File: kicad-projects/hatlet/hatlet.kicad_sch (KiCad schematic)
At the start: 29 parts, among them J1 USB Header, J2 SWD, SW1 BOOTSEL, U1 AMS1117-3.3, U2 RP2040, U3 W25Q128JVS

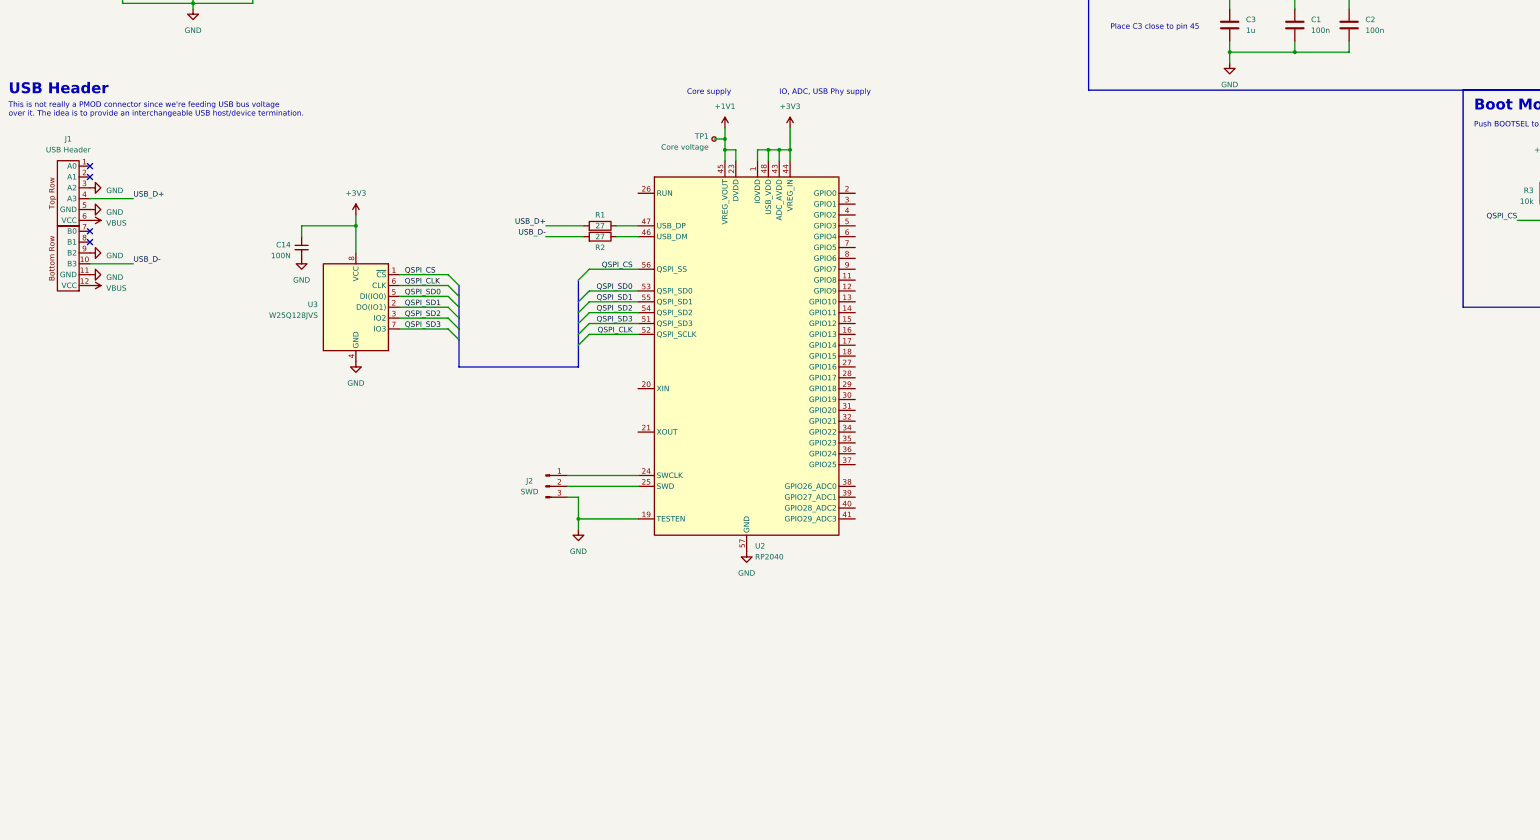
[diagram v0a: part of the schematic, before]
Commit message: Add crystal
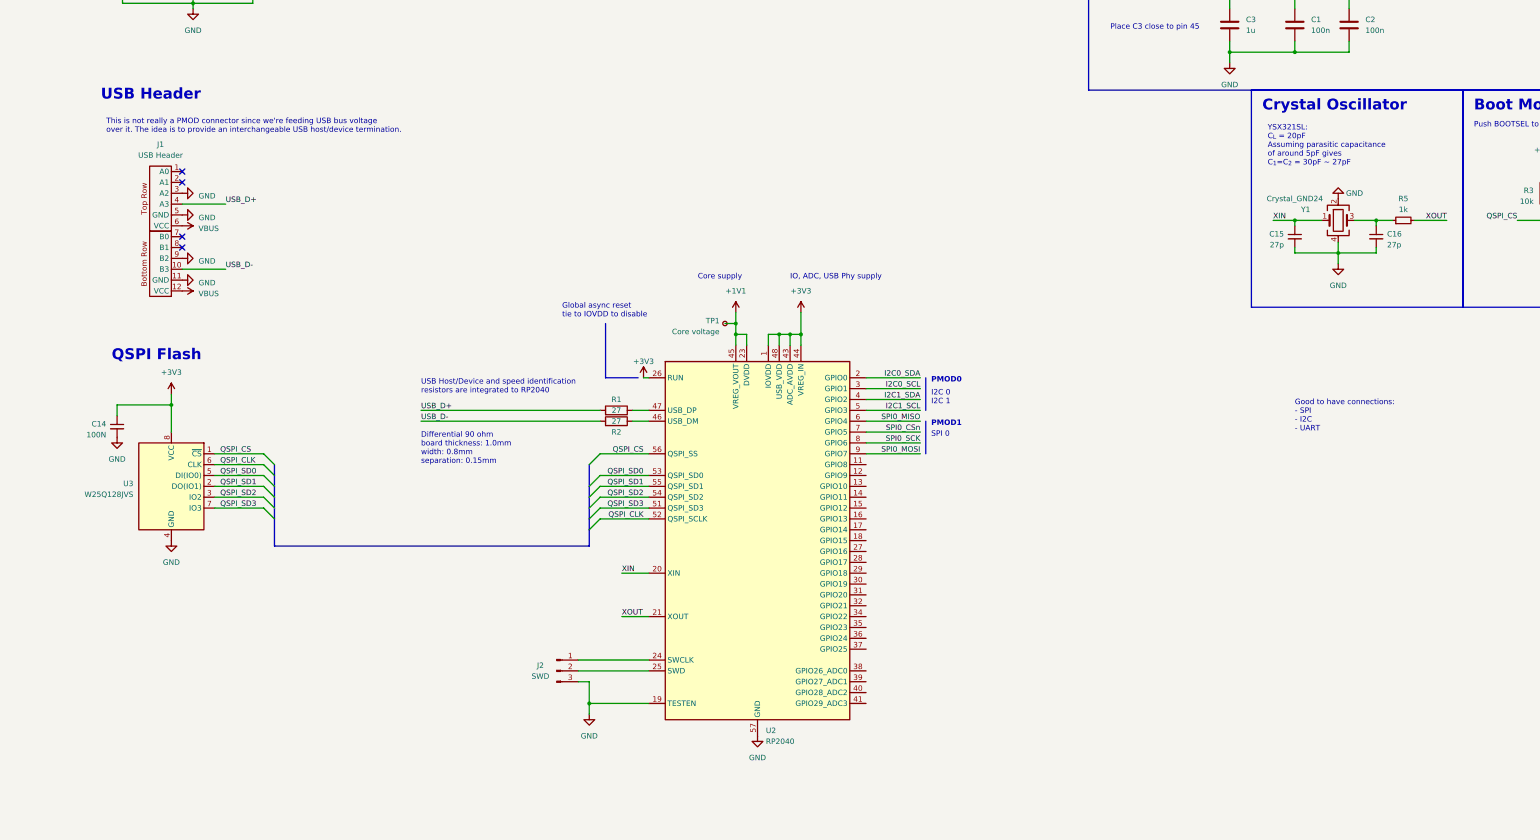
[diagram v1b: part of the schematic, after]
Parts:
- added C15, C16: 27p, symbol Device:C_Small
- added R5: 1k, symbol Device:R_Small
- added Y1: Crystal_GND24, Crystal:Crystal_SMD_3225-4Pin_3.2x2.5mm, symbol Device:Crystal_GND24
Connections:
- net +3V3: now also U2.26 (RUN)
- net GND: now also C15.2, C16.2, Y1.2, Y1.4
- net I2C0_SDA: now reaches U2.2 (GPIO0)
- net XIN: now reaches U2.20 (XIN)
- net XIN: now also C15.1, Y1.1
- net XOUT: now reaches U2.21 (XOUT)
- net XOUT: now also R5.2
- net I2C0_SCL: now reaches U2.3 (GPIO1)
- net I2C1_SDA: now reaches U2.4 (GPIO2)
- net I2C1_SCL: now reaches U2.5 (GPIO3)
- net SPI0_MISO: now reaches U2.6 (GPIO4)
- net SPI0_CSn: now reaches U2.7 (GPIO5)
- net SPI0_SCK: now reaches U2.8 (GPIO6)
- net SPI0_MOSI: now reaches U2.9 (GPIO7)
- new net: C16.1, R5.1, Y1.3
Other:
- note added: "Crystal Oscillator"
- note added: "Differential 90 ohm board thickness: 1.0mm width: 0.8mm separation: 0.15mm"
- note added: "Global async reset tie to IOVDD to disable"
- note added: "Good to have connections: - SPI - I2C - UART"
- note added: "I2C 0 I2C 1"
- note added: "PMOD0"
- note added: "PMOD1"
- note added: "QSPI Flash"
- note added: "SPI 0"
- note added: "USB Host/Device and speed identification resistors are integrated to RP2040"
- note added: "YSX321SL: C_{L} = 20pF Assuming parasitic capacitance of around 5pF gives C_{1}=C_{2} = 30pF ~ 27pF"
- moved on the sheet: C14, J1, J2, R1, R2, TP1, U2, U3
